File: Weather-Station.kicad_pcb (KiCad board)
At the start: 2 copper layers, 177.8 x 106.7 mm, 3 parts, among them J1 Conn_01x22, J2 Conn_01x22, U1 ESP32-S3-DevKitC

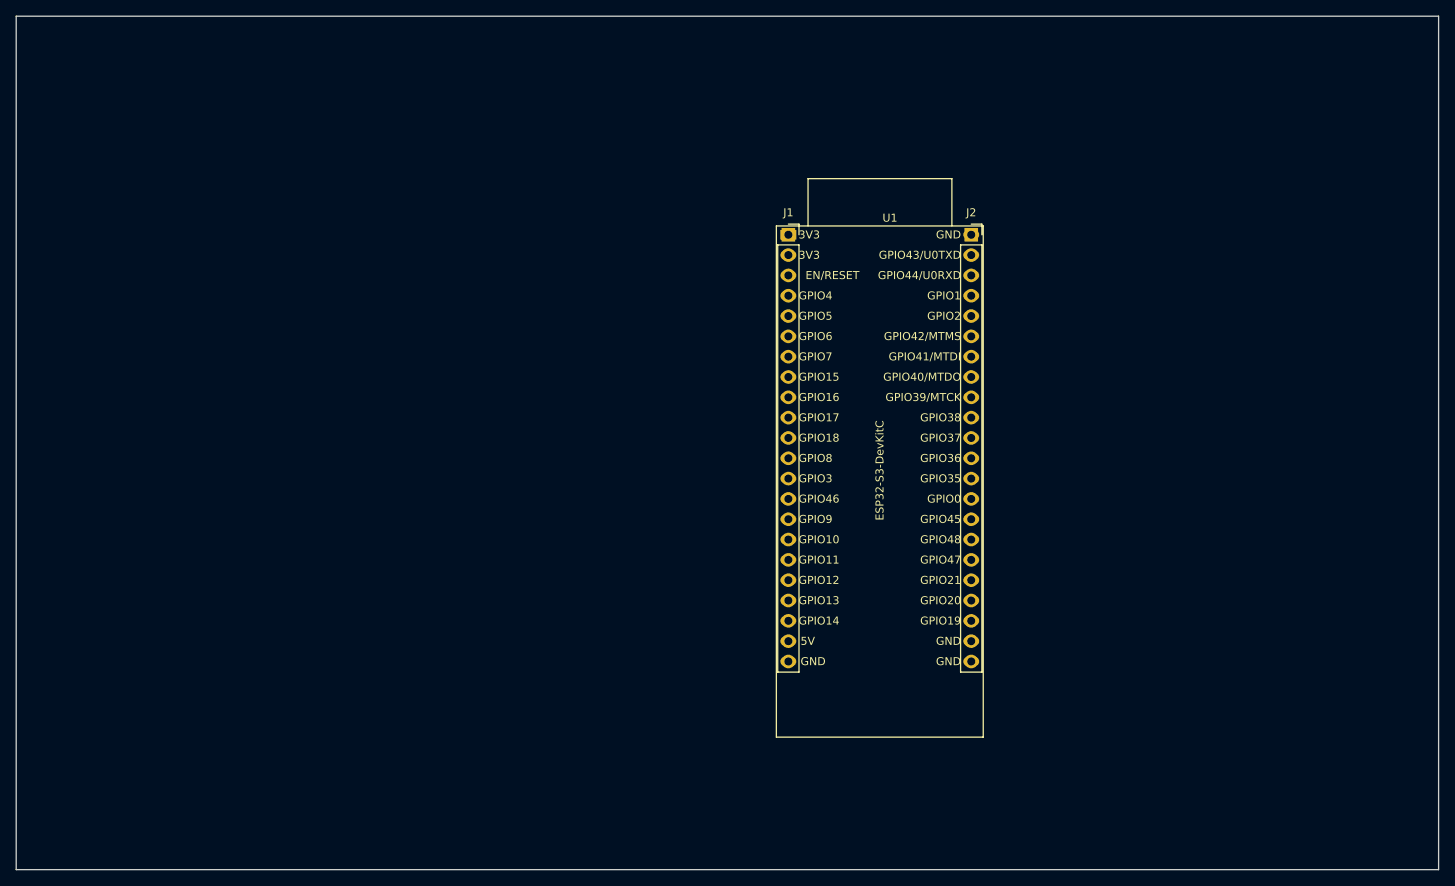
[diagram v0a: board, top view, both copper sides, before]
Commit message: WIP: Finding pin headers/rows
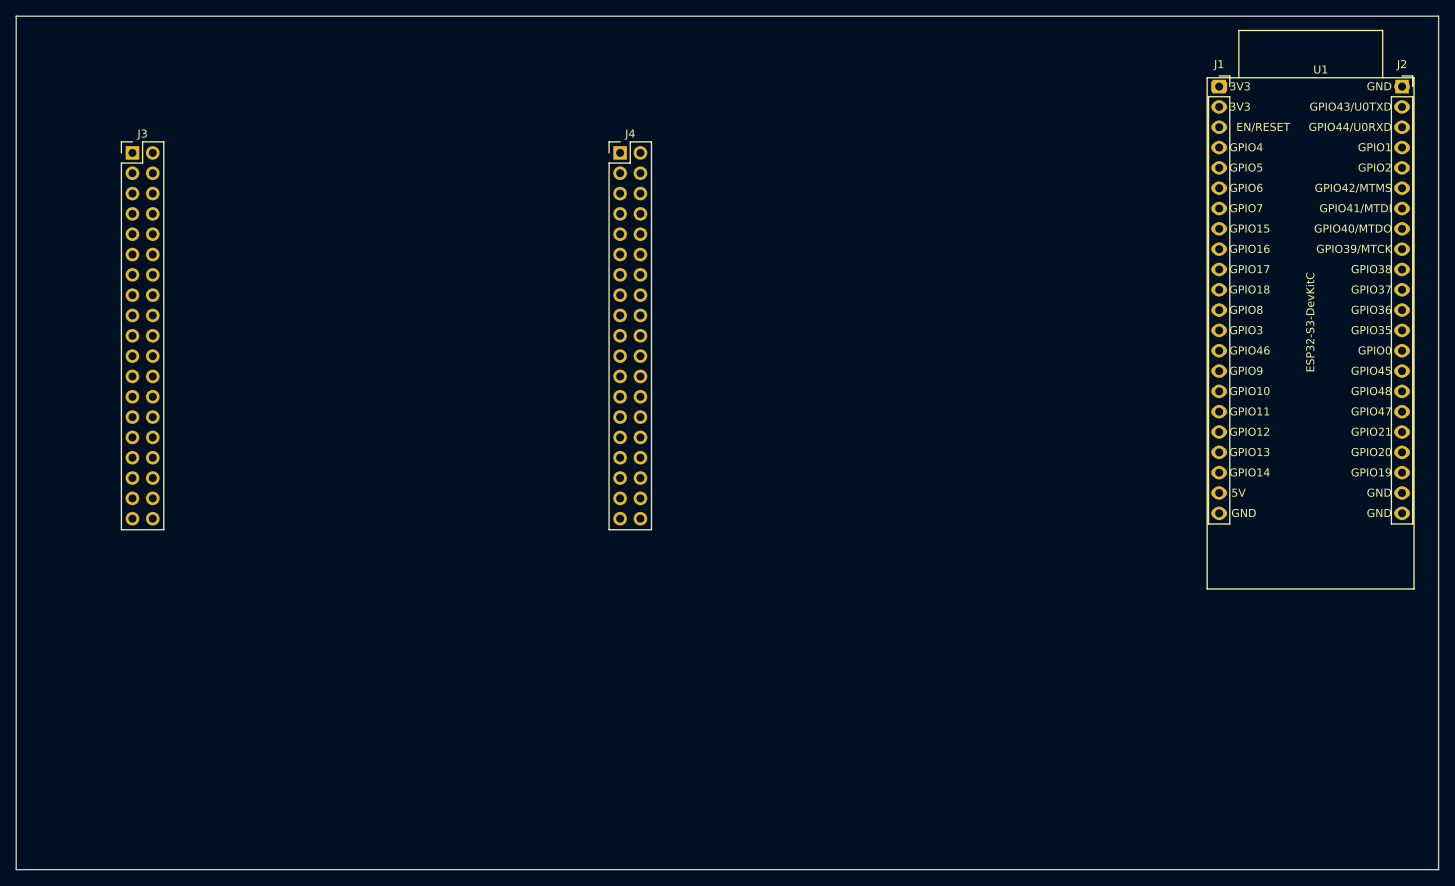
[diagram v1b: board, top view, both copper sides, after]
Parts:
- added J3: Conn_02x19_Odd_Even, Connector_PinHeader_2.54mm:PinHeader_2x19_P2.54mm_Vertical, F.Cu at (83.1, 60.3)
- added J4: Conn_02x19_Odd_Even, Connector_PinHeader_2.54mm:PinHeader_2x19_P2.54mm_Vertical, F.Cu at (144.1, 60.3)
- moved J1 56.9 mm to (218.9, 52.0)
- moved U1 56.9 mm to (218.9, 52.0)
- moved J2 56.9 mm to (241.8, 52.0)
